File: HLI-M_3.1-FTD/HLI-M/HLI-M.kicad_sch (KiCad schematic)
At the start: 115 parts, among them CON1 , CON2 USB_B, CON3 , CON4 Connector_Adapter, CON5 Connector_Audio, CON6 Conn_01x15, CON7 Conn_01x09, CON8 CR123A, Q1 DMP3068L-7, Q2 BC817, Q3 BC817, Q4 BSS84, Q5 BSS84, Q6 BSS84, Q7 BSS84, U1 PIC24HJ64GP206-I_PT, U10 24AA02-OT, U11 ULN2003, U12 ULN2003, U13 ULN2003, U2 FM25V10-GTR, U3 MAX3232, U4 TPS7A0533PDBV, U5 TPS7A0533PDBV, U6 LM3658SD, U8 FT232RL, U9 ATSHA204A-SSHDA-B, Y1 Crystal_32KHz, Y2 Crystal_20MHz

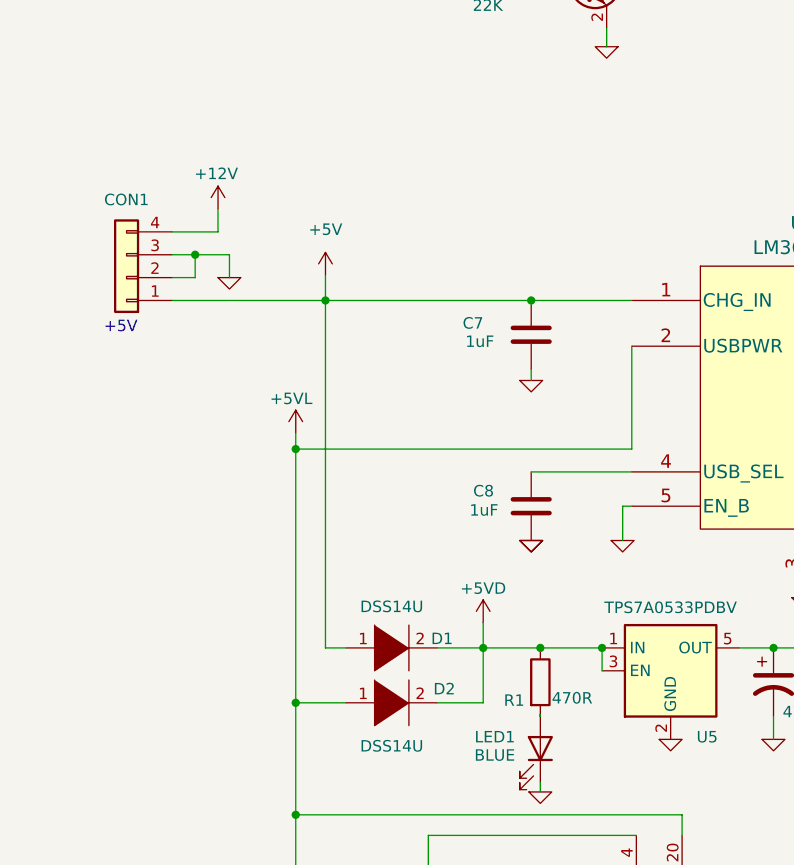
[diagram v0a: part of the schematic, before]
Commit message: att
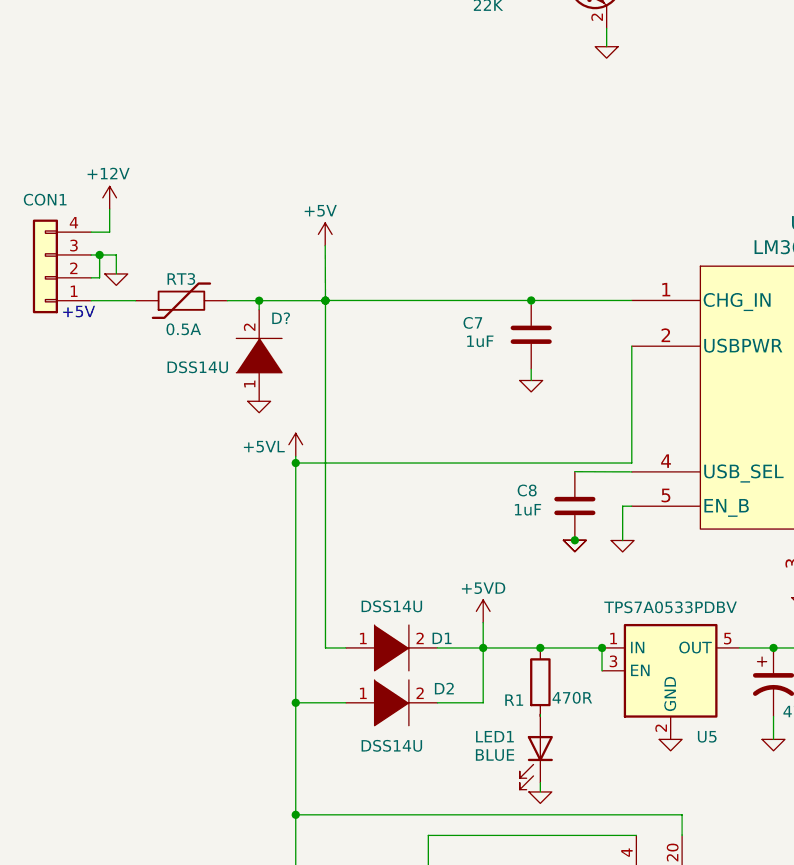
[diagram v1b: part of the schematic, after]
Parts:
- added D?: DSS14U, Diode_SMD:D_SOD-123, symbol pspice:DIODE
- added RT3: 0.5A, Resistor_SMD:R_1812_4532Metric, symbol Device:Thermistor
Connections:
- net +5V: now also D?.2 (A), RT3.2; no longer CON1.1 (Pin_1)
- net 0: now also D?.1 (K)
- new net: CON1.1 (Pin_1), RT3.1
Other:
- moved on the sheet: C8, CON1
